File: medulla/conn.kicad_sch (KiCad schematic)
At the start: 7 parts

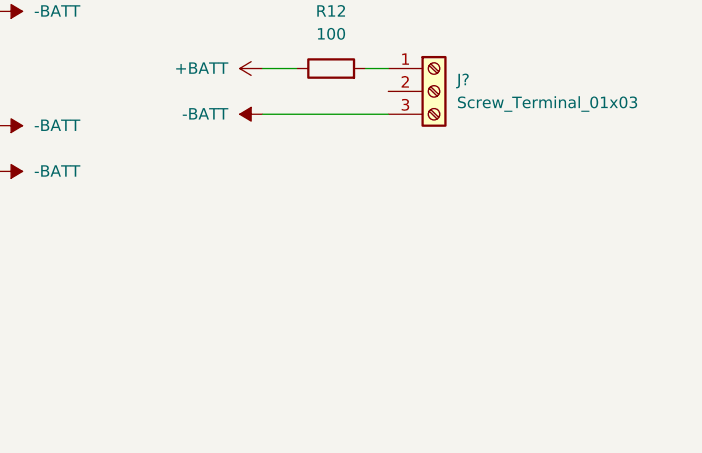
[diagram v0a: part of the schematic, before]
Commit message: 0.2.1-alpha: Minor connector changes
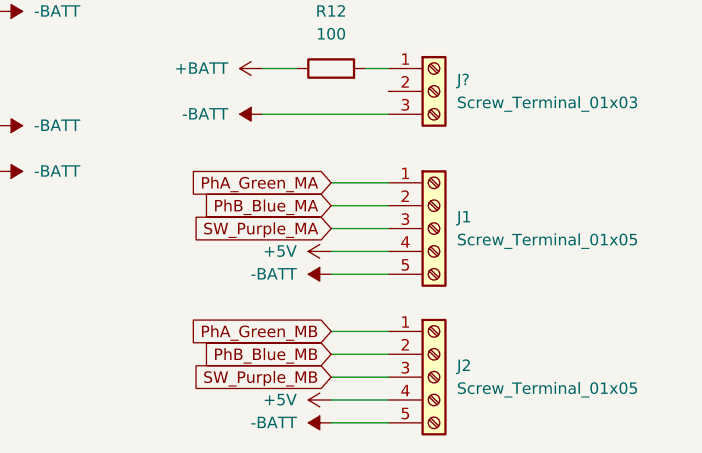
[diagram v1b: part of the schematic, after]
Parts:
- added J1, J2: Screw_Terminal_01x05, symbol Connector:Screw_Terminal_01x05
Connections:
- net +5V: now also J1.4 (Pin_4), J2.4 (Pin_4)
- net -BATT: now also J1.5 (Pin_5), J2.5 (Pin_5)
- new net PhA_Green_MA: J1.1 (Pin_1)
- new net PhA_Green_MB: J2.1 (Pin_1)
- new net PhB_Blue_MA: J1.2 (Pin_2)
- new net PhB_Blue_MB: J2.2 (Pin_2)
- new net SW_Purple_MA: J1.3 (Pin_3)
- new net SW_Purple_MB: J2.3 (Pin_3)
